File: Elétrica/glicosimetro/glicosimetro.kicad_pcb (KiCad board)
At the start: 2 copper layers, 96.2 x 67.5 mm, 20 parts, among them U1 ESP32-C3_SUPERMINI, U2 MCP6L01Rx-xOT, U3 MCP6L01Rx-xOT, U4 LM1117DT-3.3, U5 MCP6L01Rx-xOT, U6 MCP6L01Rx-xOT, U7 MCP6L01Rx-xOT

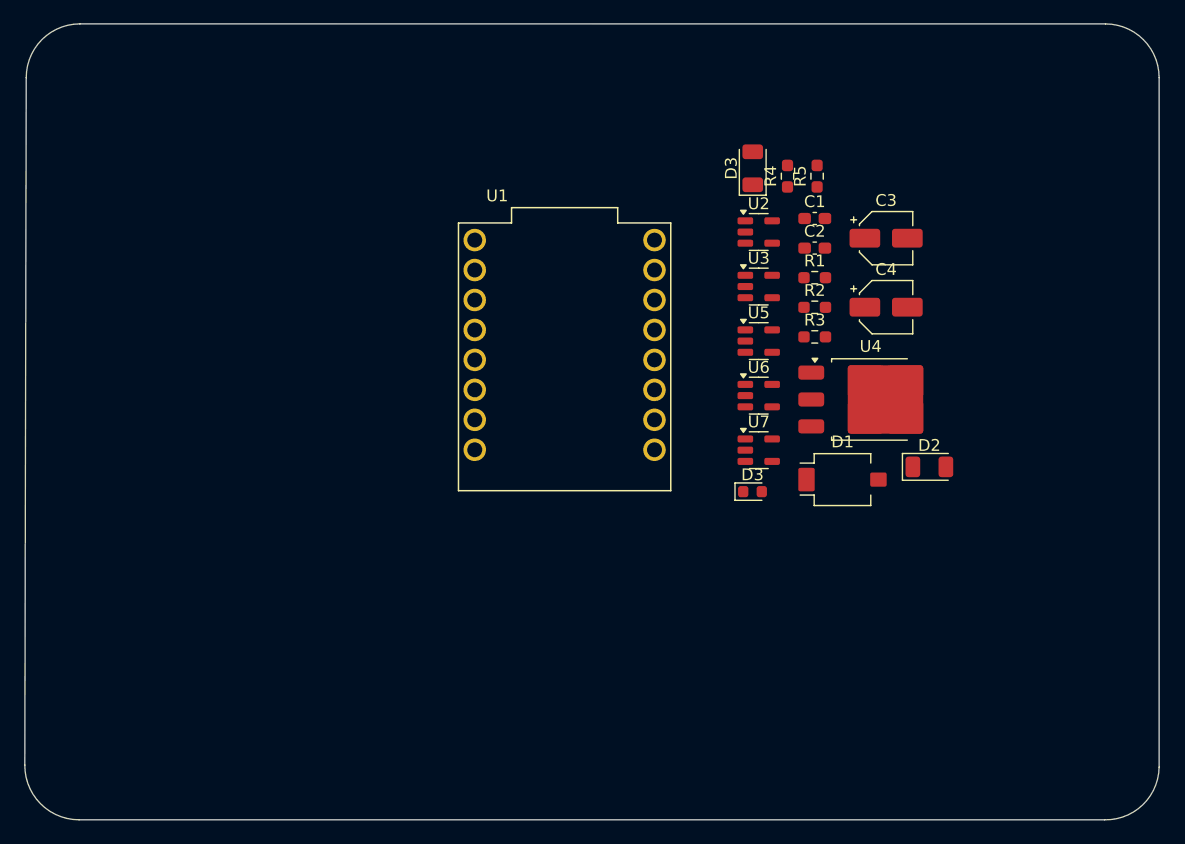
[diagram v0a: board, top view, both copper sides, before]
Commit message: Atualizações
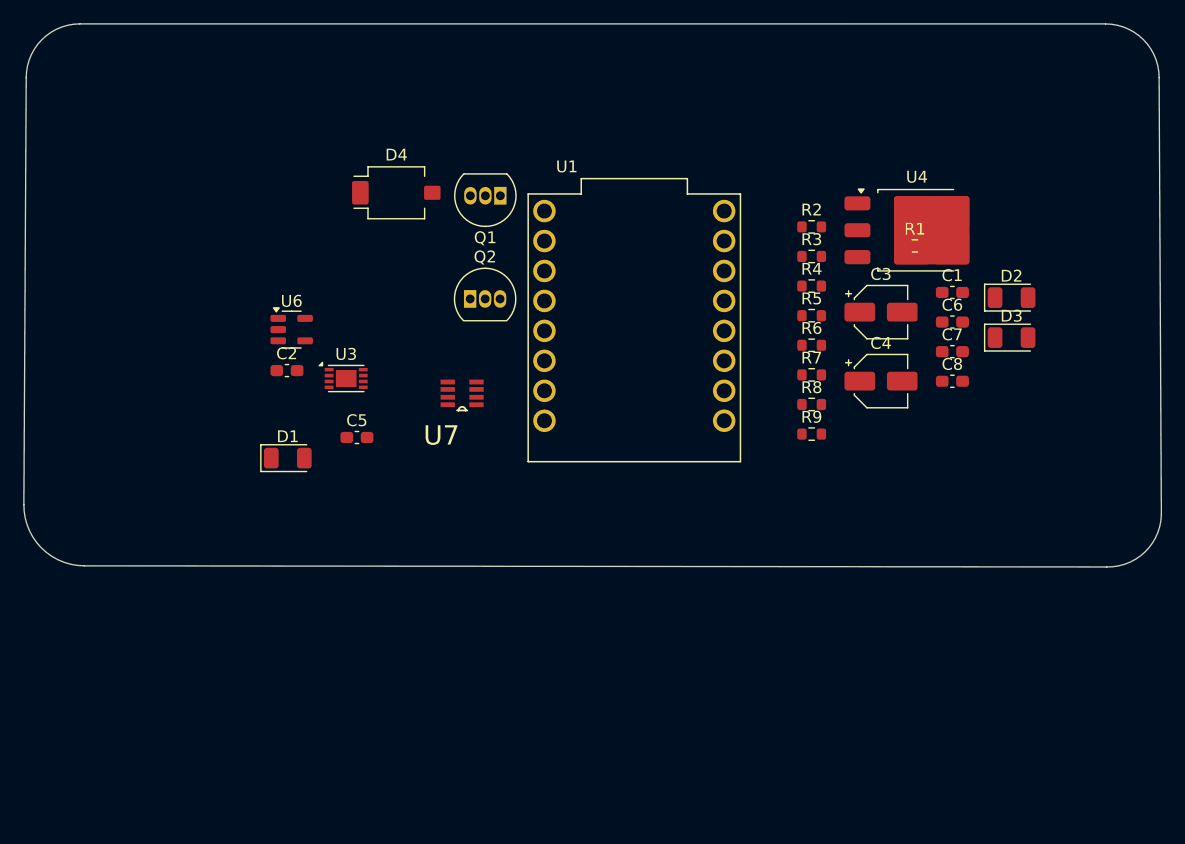
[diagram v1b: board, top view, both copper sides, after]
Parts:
- removed the D3 at (192.4, 113.3)
- removed the D3 at (192.4, 85.9)
- removed U2, U5: MCP6L01Rx-xOT, Package_TO_SOT_SMD:SOT-23-5
- added C5: 0.1uF, Capacitor_SMD:C_0603_1608Metric_Pad1.08x0.95mm_HandSolder, F.Cu at (158.9, 108.8)
- added C6: C, Capacitor_SMD:C_0603_1608Metric_Pad1.08x0.95mm_HandSolder, F.Cu at (209.3, 99.0)
- added C7: C, Capacitor_SMD:C_0603_1608Metric_Pad1.08x0.95mm_HandSolder, F.Cu at (209.3, 101.5)
- added C8: C, Capacitor_SMD:C_0603_1608Metric_Pad1.08x0.95mm_HandSolder, F.Cu at (209.3, 104.0)
- added D3: MTSM0013-844-IR 1350 nM, LED_SMD:LED_1206_3216Metric, F.Cu at (214.4, 100.3)
- added D4: S5971, OptoDevice:Osram_BPW34S-SMD, F.Cu at (162.2, 88.0)
- added Q1: BC337, Package_TO_SOT_THT:TO-92_Inline, F.Cu at (171.0, 88.2)
- added Q2: BC337, Package_TO_SOT_THT:TO-92_Inline, F.Cu at (168.5, 97.0)
- added R6: R, Resistor_SMD:R_0603_1608Metric, F.Cu at (197.4, 100.9)
- added R7: R, Resistor_SMD:R_0603_1608Metric, F.Cu at (197.4, 103.4)
- added R8: R, Resistor_SMD:R_0603_1608Metric, F.Cu at (197.4, 106.0)
- added R9: R, Resistor_SMD:R_0603_1608Metric, F.Cu at (197.4, 108.5)
- C2: value C -> 1uF
- D1: value BPW34-SMD -> MTE8120CP 805nm; footprint OptoDevice:Osram_BPW34S-SMD -> LED_SMD:LED_1206_3216Metric
- D2: value IR26-21C_L110_TR8 -> MTE8120CP 805nm
- R1, R2, R3, R4, R5: footprint Resistor_SMD:R_0603_1608Metric_Pad0.98x0.95mm_HandSolder -> Resistor_SMD:R_0603_1608Metric
- U3: value MCP6L01Rx-xOT -> MCP6002-xMC; footprint Package_TO_SOT_SMD:SOT-23-5 -> Package_DFN_QFN:DFN-8-1EP_3x2mm_P0.5mm_EP1.75x1.45mm
- U6: value MCP6L01Rx-xOT -> MCP601R
- U7: value MCP6L01Rx-xOT -> LTC6910-1CTS8PBF; footprint Package_TO_SOT_SMD:SOT-23-5 -> LTC6910-1CTS8PBF:SOT65P280X100-8N
- moved D1 47.1 mm to (153.0, 110.5)
- moved C2 45.9 mm to (152.9, 103.1)
- moved U6 40.0 mm to (153.3, 99.6)
- moved U3 35.8 mm to (157.9, 103.8)
- moved U7 25.6 mm to (167.8, 105.0), turned to 180 degrees
- moved D2 16.0 mm to (214.4, 96.9)
- moved U4 14.9 mm to (206.3, 91.2)
- moved C1 13.2 mm to (209.3, 96.5)
- moved R5 11.8 mm to (197.4, 98.4), turned to 0 degrees
- moved R4 9.54 mm to (197.4, 95.9), turned to 0 degrees
- moved R1 8.91 mm to (206.2, 92.5)
- moved R2 6.82 mm to (197.4, 90.9)
- moved R3 6.82 mm to (197.4, 93.4)
- moved U1 6.40 mm to (182.4, 99.5)
- moved C3 6.28 mm to (203.3, 98.1)
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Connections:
- C1 pad 1: Net-(D1-K) -> Net-(U3A-+)
- C2 pad 1: Net-(D1-K) -> Net-(D4-K)
- C2 pad 2: Sinal -> GND
- D1 pad 2: GND -> 3v3
- D2 pad 1: GND -> Net-(D2-K)
- D2 pad 2: Net-(D2-A) -> 3v3
- R1 pad 1: Net-(D1-K) -> Estágio3_Filtro
- R1 pad 2: Sinal -> Net-(C6-Pad1)
- R2 pad 1: GND -> Net-(D4-K)
- R2 pad 2: Net-(R2-Pad2) -> Estágio 2_Ganho
- R3 pad 1: Net-(R2-Pad2) -> Net-(C6-Pad1)
- R3 pad 2: 3v3 -> Net-(U3A-+)
- R4 pad 2: Net-(D2-A) -> Net-(Q1-B)
- U1 pad 0: unconnected-(U1-GPIO0-Pad0) -> PB - entrada AD
- U1 pad 10: unconnected-(U1-GPIO10-Pad10) -> LTC_B0
- U1 pad 20: unconnected-(U1-GPIO20-Pad20) -> LTC_B1
- U1 pad 21: unconnected-(U1-GPIO21-Pad21) -> LTC_B2
- U1 pad 3.3: unconnected-(U1-3V3-Pad3.3) -> 3v3
- U1 pad 5: unconnected-(U1-GPIO5-Pad5) -> PF - entrada AD
- U1 pad G: unconnected-(U1-GND-PadG) -> GND
- U3 pad 1: Sinal -> PB - entrada AD
- U3 pad 2: 3V3 -> GND
- U3 pad 3: REF -> Net-(U3A-+)
- U3 pad 4: Net-(D1-K) -> GND
- U6 pad 1: unconnected-(U6-Pad1) -> Estágio 2_Ganho
- U6 pad 2: unconnected-(U6-V+-Pad2) -> GND
- U6 pad 3: unconnected-(U6-+-Pad3) -> GND
- U6 pad 4: unconnected-(U6---Pad4) -> Net-(D4-K)
- U6 pad 5: unconnected-(U6-V--Pad5) -> 3v3
- U7 pad 1: unconnected-(U7-Pad1) -> Estágio3_Filtro
- U7 pad 2: unconnected-(U7-V+-Pad2) -> GND
- U7 pad 3: unconnected-(U7-+-Pad3) -> Estágio 2_Ganho
- U7 pad 4: unconnected-(U7---Pad4) -> GND
- U7 pad 5: unconnected-(U7-V--Pad5) -> LTC_B0
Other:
- board size 96.2 x 67.5 mm -> 96.5 x 46.1 mm
